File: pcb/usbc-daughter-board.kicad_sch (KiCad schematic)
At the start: 11 parts, among them J1 USBC FS 2.0, J2 JST1x04, U1 USBLC6-2SC6

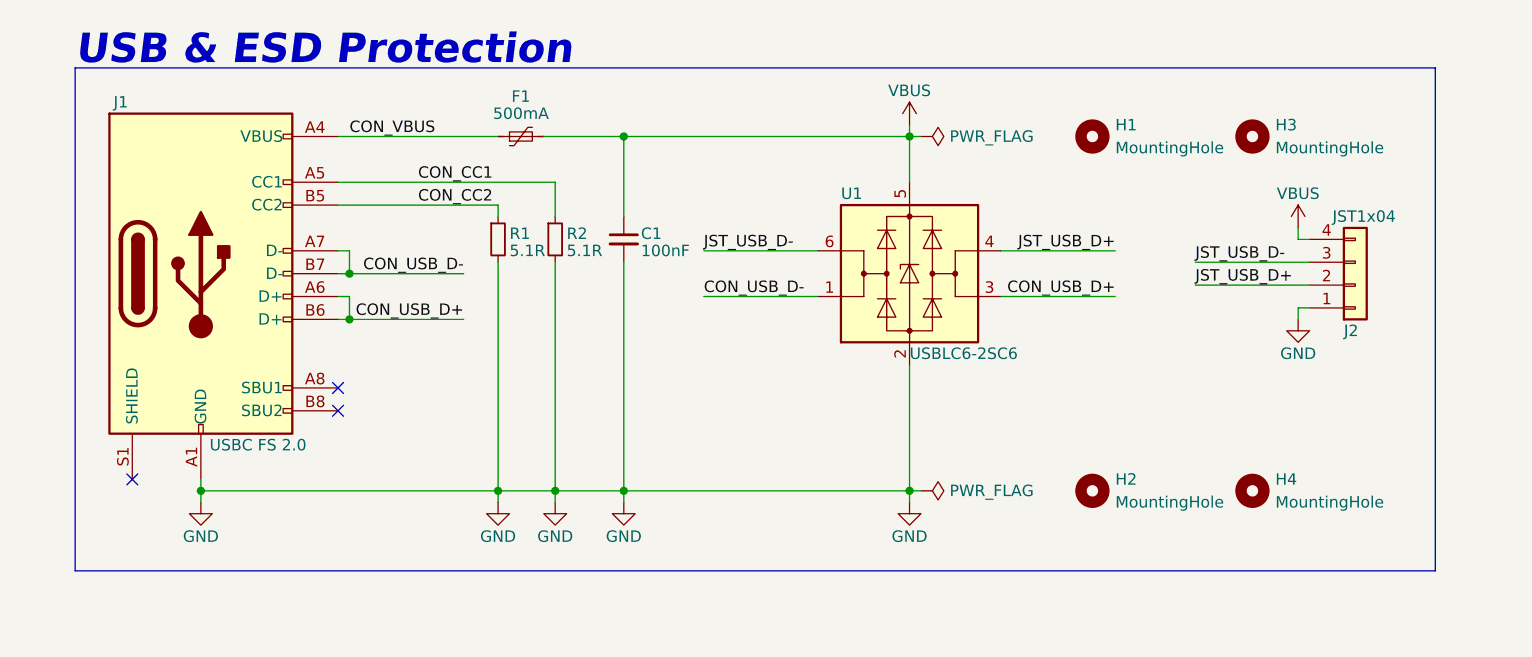
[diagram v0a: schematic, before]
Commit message: Added gerbers
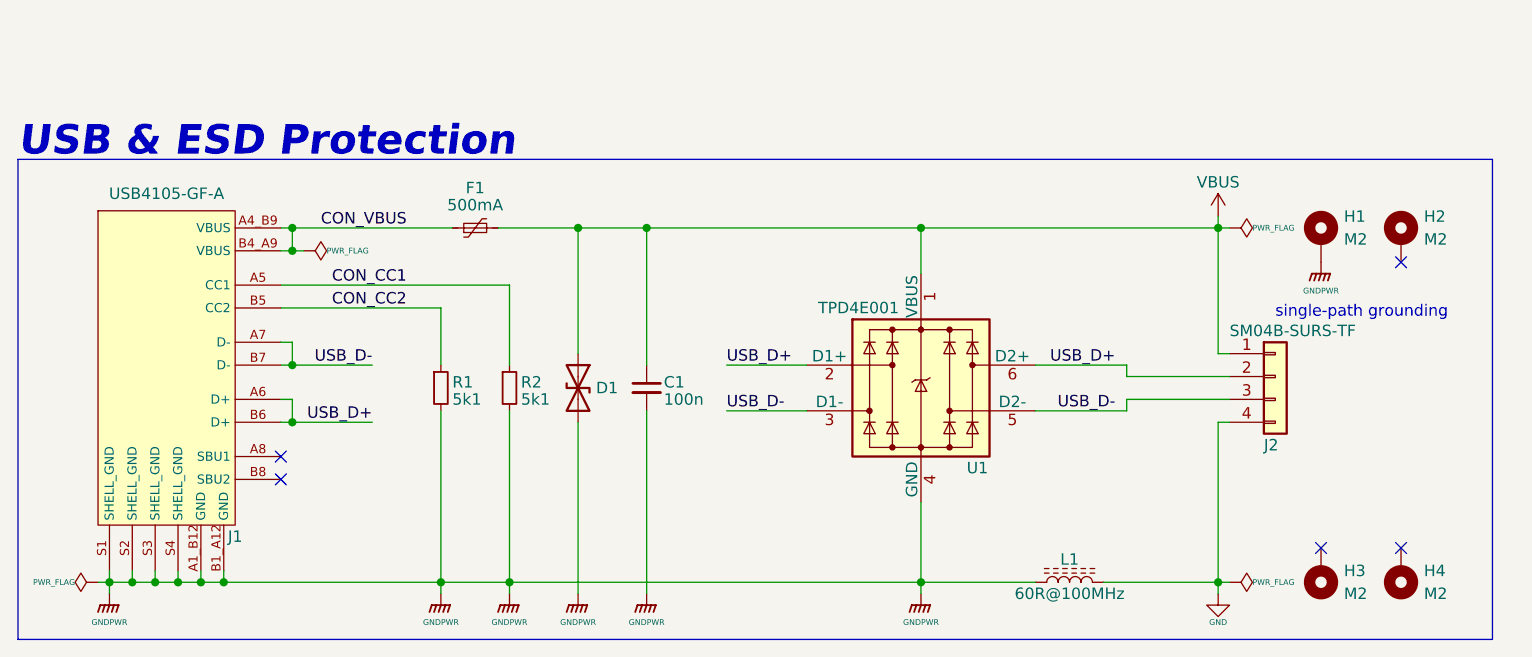
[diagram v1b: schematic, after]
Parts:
- removed H1, H2, H3, H4: MountingHole, 2mm, symbol Mechanical:MountingHole
- removed J1: USBC FS 2.0, TYPE-C-31-M-12, symbol Connector-USB-C:USB_C_Receptacle_USB2.0
- removed J2: JST1x04, SM04B-GHS-TB, symbol Connector-Generic:Conn_01x04
- removed U1: USBLC6-2SC6, SOT-23-6, symbol Power-Protection:USBLC6-2SC6
- added D1: D_TVS, Diode_SMD:D_SOD-123, symbol Device:D_TVS
- added H1, H2, H3, H4: M2, MountingHole:MountingHole_2.2mm_M2_Pad, symbol Mechanical:MountingHole_Pad
- added J1: USB4105-GF-A, Connector_USB:USB_C_Receptacle_GCT_USB4105-GF-A, symbol Connector_USB_C:USB_C_Connector
- added J2: SM04B-SURS-TF, Connector_JST:JST_SUR_SM04B-SURS-TF_1x04-1MP_P0.80mm_Horizontal, symbol Connector_Generic:Conn_01x04
- added L1: 60R@100MHz, Inductor_SMD:L_0603_1608Metric, symbol Device:L_Ferrite
- added U1: TPD4E001, Package_TO_SOT_SMD:SOT-23-6, symbol Power_Protection:TPD4E001QDBVRQ1
- C1: value 100nF -> 100n; footprint C-0603 -> Capacitor_SMD:C_0603_1608Metric; Digikey Part # (none) -> 1276-1935-1-ND; Manufacturer YAGEO -> Samsung Electro-Mechanics; Manufacturer Part # CC0603KRX7R9BB104 -> CL10B104KB8NNWC; Mouser Part # (none) -> 80-C603C104K5RAC3121
- F1: footprint F-0603 -> Fuse:Fuse_0603_1608Metric; Digikey Part # (none) -> F3733CT-ND; Manufacturer BHFUSE -> Littelfuse Inc.; Manufacturer Part # BSMD0603-050-6V -> 1206L050/15YR; Mouser Part # (none) -> 576-1206L050/15YR
- R1, R2: value 5.1R -> 5k1; footprint R-0603 -> Resistor_SMD:R_0603_1608Metric; Digikey Part # (none) -> RMCF0603FT5K10CT-ND; Manufacturer UNI-ROYAL(Uniroyal Elec) -> Stackpole Electronics Inc.; Manufacturer Part # 0603WAF5101T5E -> RMCF0603FT5K10
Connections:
- net CON_CC1: now also J1.A5 (CC1)
- net CON_CC2: now also J1.B5 (CC2)
- net CON_VBUS: now also J1.A4_B9 (VBUS), J1.B4_A9 (VBUS)
- net GND: now also J2.4 (Pin_4), L1.2; no longer C1.2, R1.2, R2.2
- net VBUS: now also D1.1 (A1), J2.1 (Pin_1), U1.1 (VBUS)
- new net GNDPWR: C1.2, D1.2 (A2), H1.1, J1.A1_B12 (GND), J1.B1_A12 (GND), J1.S1 (SHELL_GND), J1.S2 (SHELL_GND), J1.S3 (SHELL_GND), J1.S4 (SHELL_GND), L1.1, R1.2, R2.2, U1.4 (GND)
- new net USB_D+: J1.A6 (D+), J1.B6 (D+), J2.2 (Pin_2), U1.2 (D1+), U1.6 (D2+)
- new net USB_D-: J1.A7 (D-), J1.B7 (D-), J2.3 (Pin_3), U1.3 (D1-), U1.5 (D2-)
- no-connect marks 3 -> 5
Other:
- note added: "single-path grounding"
